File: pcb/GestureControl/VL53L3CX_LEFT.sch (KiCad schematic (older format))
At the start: 6 parts, among them U5 VL53L3CXV0DH_LEFT

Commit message: add
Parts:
- C12, C13: footprint Capacitor_SMD:C_0805_2012Metric_Pad1.18x1.45mm_HandSolder -> Capacitor_SMD:C_0603_1608Metric_Pad1.08x0.95mm_HandSolder
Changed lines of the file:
@@
 F 0 "C13" H 6915 3796 50  0000 L CNN
 F 1 "100n" H 6915 3705 50  0000 L CNN
-F 2 "Capacitor_SMD:C_0805_2012Metric_Pad1.18x1.45mm_HandSolder" H 6838 3600 50  0001 C CNN
+F 2 "Capacitor_SMD:C_0603_1608Metric_Pad1.08x0.95mm_HandSolder" H 6838 3600 50  0001 C CNN
 F 3 "~" H 6800 3750 50  0001 C CNN
 	1    6800 3750
@@
 F 0 "C12" H 3465 3796 50  0000 L CNN
 F 1 "100n" H 3465 3705 50  0000 L CNN
-F 2 "Capacitor_SMD:C_0805_2012Metric_Pad1.18x1.45mm_HandSolder" H 3388 3600 50  0001 C CNN
+F 2 "Capacitor_SMD:C_0603_1608Metric_Pad1.08x0.95mm_HandSolder" H 3388 3600 50  0001 C CNN
 F 3 "~" H 3350 3750 50  0001 C CNN
 	1    3350 3750

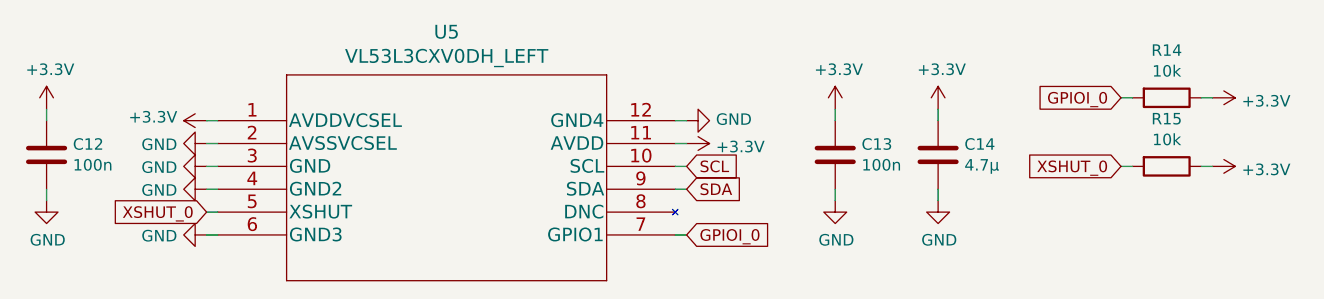
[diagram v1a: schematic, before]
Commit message: new PCB
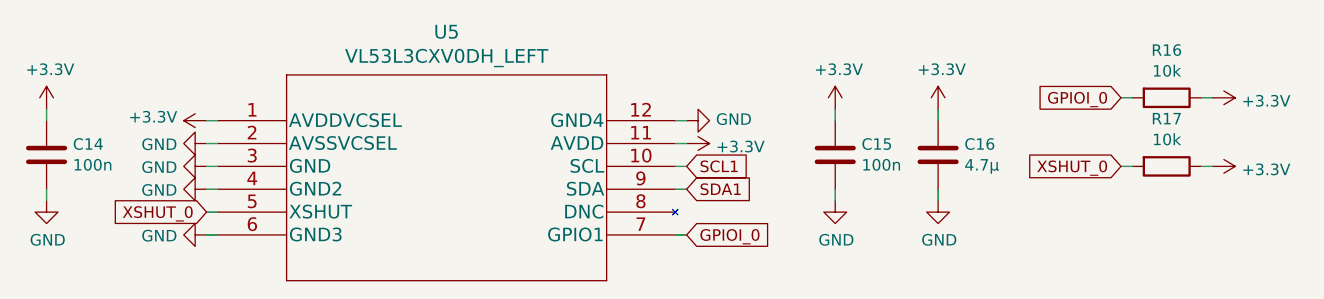
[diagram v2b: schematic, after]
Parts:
- U5: footprint VL53L3CX:VL53L3CXV0DH&slash_1 -> VL53L3C1:VL53L3CXV0DH&slash_1
- renumbered C12 to C14, C13 to C15, C14 to C16, R14 to R16, R15 to R17
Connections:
- net SCL renamed SCL1
- net SDA renamed SDA1
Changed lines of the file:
@@
 F 0 "U5" H 5100 3987 60  0000 C CNN
 F 1 "VL53L3CXV0DH_LEFT" H 5100 3881 60  0000 C CNN
-F 2 "VL53L3CX:VL53L3CXV0DH&slash_1" H 5100 3840 60  0001 C CNN
+F 2 "VL53L3C1:VL53L3CXV0DH&slash_1" H 5100 3840 60  0001 C CNN
 F 3 "" H 4100 3600 60  0000 C CNN
 	1    4100 3600
@@
 P 6150 3700
 AR Path="/62398514/623AF08A" Ref="#PWR?"  Part="1"
-AR Path="/623A3BAC/623AF08A" Ref="#PWR0147"  Part="1"
-F 0 "#PWR0147" H 6150 3550 50  0001 C CNN
+AR Path="/623A3BAC/623AF08A" Ref="#PWR059"  Part="1"
+F 0 "#PWR059" H 6150 3550 50  0001 C CNN
 F 1 "+3.3V" V 6165 3828 50  0000 L CNN
 F 2 "" H 6150 3700 50  0001 C CNN
@@
 P 6150 3600
 AR Path="/62398514/623AF090" Ref="#PWR?"  Part="1"
-AR Path="/623A3BAC/623AF090" Ref="#PWR0148"  Part="1"
-F 0 "#PWR0148" H 6150 3350 50  0001 C CNN
+AR Path="/623A3BAC/623AF090" Ref="#PWR058"  Part="1"
+F 0 "#PWR058" H 6150 3350 50  0001 C CNN
 F 1 "GND" V 6155 3472 50  0000 R CNN
 F 2 "" H 6150 3600 50  0001 C CNN
@@
 $EndComp
 Text GLabel 6150 3800 2    50   Input ~ 0
-SCL
+SCL1
 Text GLabel 6150 3900 2    50   Input ~ 0
-SDA
+SDA1
 $Comp
 L power:+3.3V #PWR?
@@
 P 4050 3600
 AR Path="/62398514/623AF098" Ref="#PWR?"  Part="1"
-AR Path="/623A3BAC/623AF098" Ref="#PWR0149"  Part="1"
-F 0 "#PWR0149" H 4050 3450 50  0001 C CNN
+AR Path="/623A3BAC/623AF098" Ref="#PWR053"  Part="1"
+F 0 "#PWR053" H 4050 3450 50  0001 C CNN
 F 1 "+3.3V" V 4065 3728 50  0000 L CNN
 F 2 "" H 4050 3600 50  0001 C CNN
@@
 P 4050 3800
 AR Path="/62398514/623AF09E" Ref="#PWR?"  Part="1"
-AR Path="/623A3BAC/623AF09E" Ref="#PWR0150"  Part="1"
-F 0 "#PWR0150" H 4050 3550 50  0001 C CNN
+AR Path="/623A3BAC/623AF09E" Ref="#PWR055"  Part="1"
+F 0 "#PWR055" H 4050 3550 50  0001 C CNN
 F 1 "GND" V 4055 3672 50  0000 R CNN
 F 2 "" H 4050 3800 50  0001 C CNN
@@
 P 4050 3900
 AR Path="/62398514/623AF0A4" Ref="#PWR?"  Part="1"
-AR Path="/623A3BAC/623AF0A4" Ref="#PWR0151"  Part="1"
-F 0 "#PWR0151" H 4050 3650 50  0001 C CNN
+AR Path="/623A3BAC/623AF0A4" Ref="#PWR056"  Part="1"
+F 0 "#PWR056" H 4050 3650 50  0001 C CNN
 F 1 "GND" V 4055 3772 50  0000 R CNN
 F 2 "" H 4050 3900 50  0001 C CNN
@@
 P 4050 4100
 AR Path="/62398514/623AF0AA" Ref="#PWR?"  Part="1"
-AR Path="/623A3BAC/623AF0AA" Ref="#PWR0152"  Part="1"
-F 0 "#PWR0152" H 4050 3850 50  0001 C CNN
+AR Path="/623A3BAC/623AF0AA" Ref="#PWR057"  Part="1"
+F 0 "#PWR057" H 4050 3850 50  0001 C CNN
 F 1 "GND" V 4055 3972 50  0000 R CNN
 F 2 "" H 4050 4100 50  0001 C CNN
@@
 P 4050 3700
 AR Path="/62398514/623AF0B1" Ref="#PWR?"  Part="1"
-AR Path="/623A3BAC/623AF0B1" Ref="#PWR0153"  Part="1"
-F 0 "#PWR0153" H 4050 3450 50  0001 C CNN
+AR Path="/623A3BAC/623AF0B1" Ref="#PWR054"  Part="1"
+F 0 "#PWR054" H 4050 3450 50  0001 C CNN
 F 1 "GND" V 4055 3572 50  0000 R CNN
 F 2 "" H 4050 3700 50  0001 C CNN
@@
 P 6800 3750
 AR Path="/62398514/623AF0C2" Ref="C?"  Part="1"
-AR Path="/623A3BAC/623AF0C2" Ref="C13"  Part="1"
-F 0 "C13" H 6915 3796 50  0000 L CNN
+AR Path="/623A3BAC/623AF0C2" Ref="C15"  Part="1"
+F 0 "C15" H 6915 3796 50  0000 L CNN
 F 1 "100n" H 6915 3705 50  0000 L CNN
 F 2 "Capacitor_SMD:C_0603_1608Metric_Pad1.08x0.95mm_HandSolder" H 6838 3600 50  0001 C CNN
@@
 P 7250 3750
 AR Path="/62398514/623AF0C8" Ref="C?"  Part="1"
-AR Path="/623A3BAC/623AF0C8" Ref="C14"  Part="1"
-F 0 "C14" H 7365 3796 50  0000 L CNN
+AR Path="/623A3BAC/623AF0C8" Ref="C16"  Part="1"
+F 0 "C16" H 7365 3796 50  0000 L CNN
 F 1 "4.7µ" H 7365 3705 50  0000 L CNN
 F 2 "Capacitor_SMD:C_0805_2012Metric_Pad1.18x1.45mm_HandSolder" H 7288 3600 50  0001 C CNN
@@
 P 6800 3550
 AR Path="/62398514/623AF0CE" Ref="#PWR?"  Part="1"
-AR Path="/623A3BAC/623AF0CE" Ref="#PWR0154"  Part="1"
-F 0 "#PWR0154" H 6800 3400 50  0001 C CNN
+AR Path="/623A3BAC/623AF0CE" Ref="#PWR060"  Part="1"
+F 0 "#PWR060" H 6800 3400 50  0001 C CNN
 F 1 "+3.3V" H 6815 3723 50  0000 C CNN
 F 2 "" H 6800 3550 50  0001 C CNN
@@
 P 7250 3550
 AR Path="/62398514/623AF0D4" Ref="#PWR?"  Part="1"
-AR Path="/623A3BAC/623AF0D4" Ref="#PWR0155"  Part="1"
-F 0 "#PWR0155" H 7250 3400 50  0001 C CNN
+AR Path="/623A3BAC/623AF0D4" Ref="#PWR062"  Part="1"
+F 0 "#PWR062" H 7250 3400 50  0001 C CNN
 F 1 "+3.3V" H 7265 3723 50  0000 C CNN
 F 2 "" H 7250 3550 50  0001 C CNN
@@
 P 6800 3950
 AR Path="/62398514/623AF0DA" Ref="#PWR?"  Part="1"
-AR Path="/623A3BAC/623AF0DA" Ref="#PWR0156"  Part="1"
-F 0 "#PWR0156" H 6800 3700 50  0001 C CNN
+AR Path="/623A3BAC/623AF0DA" Ref="#PWR061"  Part="1"
+F 0 "#PWR061" H 6800 3700 50  0001 C CNN
 F 1 "GND" H 6805 3777 50  0000 C CNN
 F 2 "" H 6800 3950 50  0001 C CNN
@@
 P 7250 3950
 AR Path="/62398514/623AF0E0" Ref="#PWR?"  Part="1"
-AR Path="/623A3BAC/623AF0E0" Ref="#PWR0157"  Part="1"
-F 0 "#PWR0157" H 7250 3700 50  0001 C CNN
+AR Path="/623A3BAC/623AF0E0" Ref="#PWR063"  Part="1"
+F 0 "#PWR063" H 7250 3700 50  0001 C CNN
 F 1 "GND" H 7255 3777 50  0000 C CNN
 F 2 "" H 7250 3950 50  0001 C CNN
@@
 P 8250 3800
 AR Path="/62398514/623AF0E6" Ref="R?"  Part="1"
-AR Path="/623A3BAC/623AF0E6" Ref="R15"  Part="1"
-F 0 "R15" V 8043 3800 50  0000 C CNN
+AR Path="/623A3BAC/623AF0E6" Ref="R17"  Part="1"
+F 0 "R17" V 8043 3800 50  0000 C CNN
 F 1 "10k" V 8134 3800 50  0000 C CNN
 F 2 "Resistor_SMD:R_0805_2012Metric_Pad1.20x1.40mm_HandSolder" V 8180 3800 50  0001 C CNN
@@
 P 8250 3500
 AR Path="/62398514/623AF0EC" Ref="R?"  Part="1"
-AR Path="/623A3BAC/623AF0EC" Ref="R14"  Part="1"
-F 0 "R14" V 8043 3500 50  0000 C CNN
+AR Path="/623A3BAC/623AF0EC" Ref="R16"  Part="1"
+F 0 "R16" V 8043 3500 50  0000 C CNN
 F 1 "10k" V 8134 3500 50  0000 C CNN
 F 2 "Resistor_SMD:R_0805_2012Metric_Pad1.20x1.40mm_HandSolder" V 8180 3500 50  0001 C CNN
@@
 P 8450 3500
 AR Path="/62398514/623AF0F4" Ref="#PWR?"  Part="1"
-AR Path="/623A3BAC/623AF0F4" Ref="#PWR0158"  Part="1"
-F 0 "#PWR0158" H 8450 3350 50  0001 C CNN
+AR Path="/623A3BAC/623AF0F4" Ref="#PWR064"  Part="1"
+F 0 "#PWR064" H 8450 3350 50  0001 C CNN
 F 1 "+3.3V" V 8465 3628 50  0000 L CNN
 F 2 "" H 8450 3500 50  0001 C CNN
@@
 P 8450 3800
 AR Path="/62398514/623AF0FA" Ref="#PWR?"  Part="1"
-AR Path="/623A3BAC/623AF0FA" Ref="#PWR0159"  Part="1"
-F 0 "#PWR0159" H 8450 3650 50  0001 C CNN
+AR Path="/623A3BAC/623AF0FA" Ref="#PWR065"  Part="1"
+F 0 "#PWR065" H 8450 3650 50  0001 C CNN
 F 1 "+3.3V" V 8465 3928 50  0000 L CNN
 F 2 "" H 8450 3800 50  0001 C CNN
@@
 P 3350 3750
 AR Path="/62398514/623AF108" Ref="C?"  Part="1"
-AR Path="/623A3BAC/623AF108" Ref="C12"  Part="1"
-F 0 "C12" H 3465 3796 50  0000 L CNN
+AR Path="/623A3BAC/623AF108" Ref="C14"  Part="1"
+F 0 "C14" H 3465 3796 50  0000 L CNN
 F 1 "100n" H 3465 3705 50  0000 L CNN
 F 2 "Capacitor_SMD:C_0603_1608Metric_Pad1.08x0.95mm_HandSolder" H 3388 3600 50  0001 C CNN
@@
 P 3350 3550
 AR Path="/62398514/623AF10E" Ref="#PWR?"  Part="1"
-AR Path="/623A3BAC/623AF10E" Ref="#PWR0160"  Part="1"
-F 0 "#PWR0160" H 3350 3400 50  0001 C CNN
+AR Path="/623A3BAC/623AF10E" Ref="#PWR051"  Part="1"
+F 0 "#PWR051" H 3350 3400 50  0001 C CNN
 F 1 "+3.3V" H 3365 3723 50  0000 C CNN
 F 2 "" H 3350 3550 50  0001 C CNN
@@
 P 3350 3950
 AR Path="/62398514/623AF114" Ref="#PWR?"  Part="1"
-AR Path="/623A3BAC/623AF114" Ref="#PWR0161"  Part="1"
-F 0 "#PWR0161" H 3350 3700 50  0001 C CNN
+AR Path="/623A3BAC/623AF114" Ref="#PWR052"  Part="1"
+F 0 "#PWR052" H 3350 3700 50  0001 C CNN
 F 1 "GND" H 3355 3777 50  0000 C CNN
 F 2 "" H 3350 3950 50  0001 C CNN

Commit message: add lib inside PCB
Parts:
- U5: footprint VL53L3C1:VL53L3CXV0DH&slash_1 -> VL53L3CX:VL53L3CXV0DH&slash_1
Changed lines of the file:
@@
 AR Path="/62398514/623AF083" Ref="U?"  Part="1"
 AR Path="/623A3BAC/623AF083" Ref="U5"  Part="1"
+AR Path="/623AF083" Ref="U5"  Part="1"
 F 0 "U5" H 5100 3987 60  0000 C CNN
 F 1 "VL53L3CXV0DH_LEFT" H 5100 3881 60  0000 C CNN
-F 2 "VL53L3C1:VL53L3CXV0DH&slash_1" H 5100 3840 60  0001 C CNN
+F 2 "VL53L3CX:VL53L3CXV0DH&slash_1" H 5100 3840 60  0001 C CNN
 F 3 "" H 4100 3600 60  0000 C CNN
 	1    4100 3600

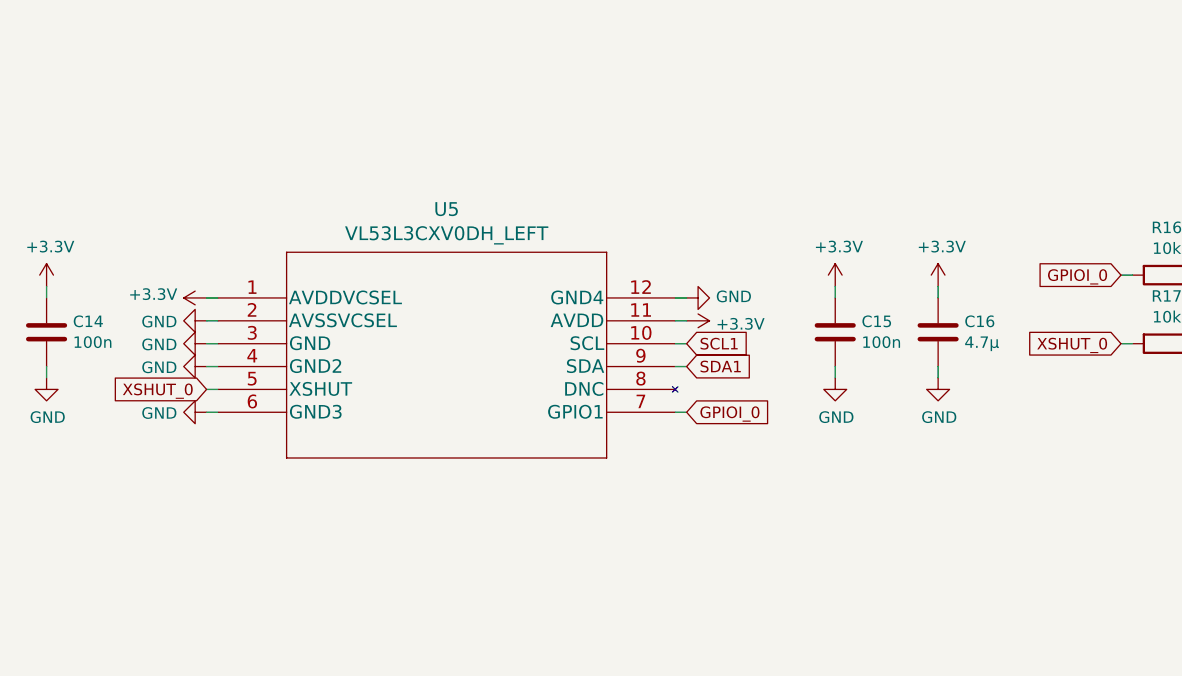
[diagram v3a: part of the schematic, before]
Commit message: add feedback Philip
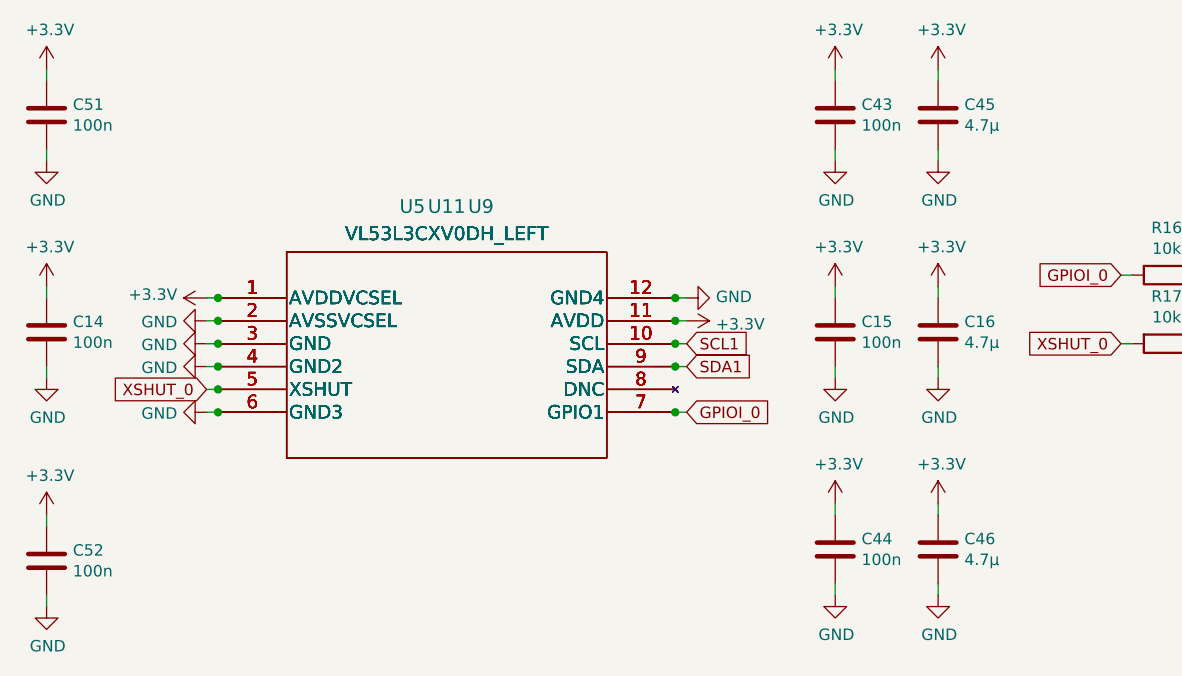
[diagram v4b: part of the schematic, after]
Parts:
- added C43, C44, C51, C52: 100n, Capacitor_SMD:C_0603_1608Metric_Pad1.08x0.95mm_HandSolder, symbol Device:C
- added C45, C46: 4.7µ, Capacitor_SMD:C_0805_2012Metric_Pad1.18x1.45mm_HandSolder, symbol Device:C
- added U11, U9: VL53L3CXV0DH_LEFT, VL53L3CX:VL53L3CXV0DH&slash_1, symbol VL53L3CX:VL53L3CXV0DH_1
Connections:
- net +3V3: now also C43.1, C44.1, C45.1, C46.1, C51.1, C52.1, U11.1 (AVDDVCSEL), U11.11 (AVDD), U9.1 (AVDDVCSEL), U9.11 (AVDD)
- net GND: now also C43.2, C44.2, C45.2, C46.2, C51.2, C52.2, U11.12 (GND4), U11.2 (AVSSVCSEL), U11.3 (GND), U11.4 (GND2), U11.6 (GND3), U9.12 (GND4), U9.2 (AVSSVCSEL), U9.3 (GND), U9.4 (GND2), U9.6 (GND3)
- net GPIOI_0: now also U11.7 (GPIO1), U9.7 (GPIO1)
- net SCL1: now also U11.10 (SCL), U9.10 (SCL)
- net SDA1: now also U11.9 (SDA), U9.9 (SDA)
- net XSHUT_0: now also U11.5 (XSHUT), U9.5 (XSHUT)
- net at U5.8 (DNC): now also U11.8 (DNC), U9.8 (DNC)

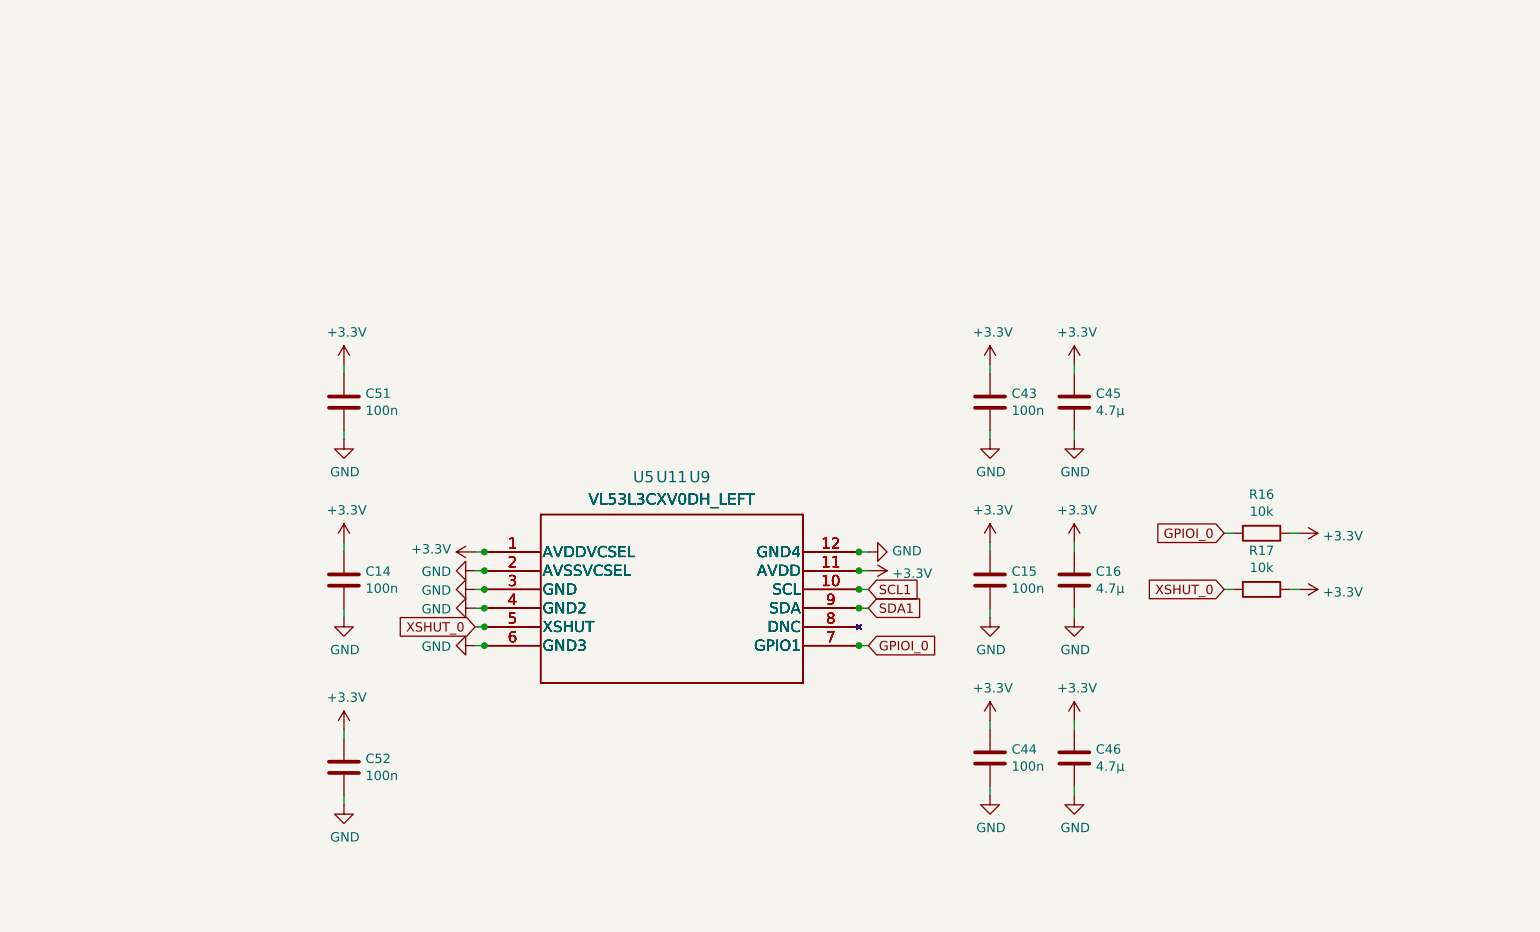
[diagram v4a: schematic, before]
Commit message: add PCBV0.11
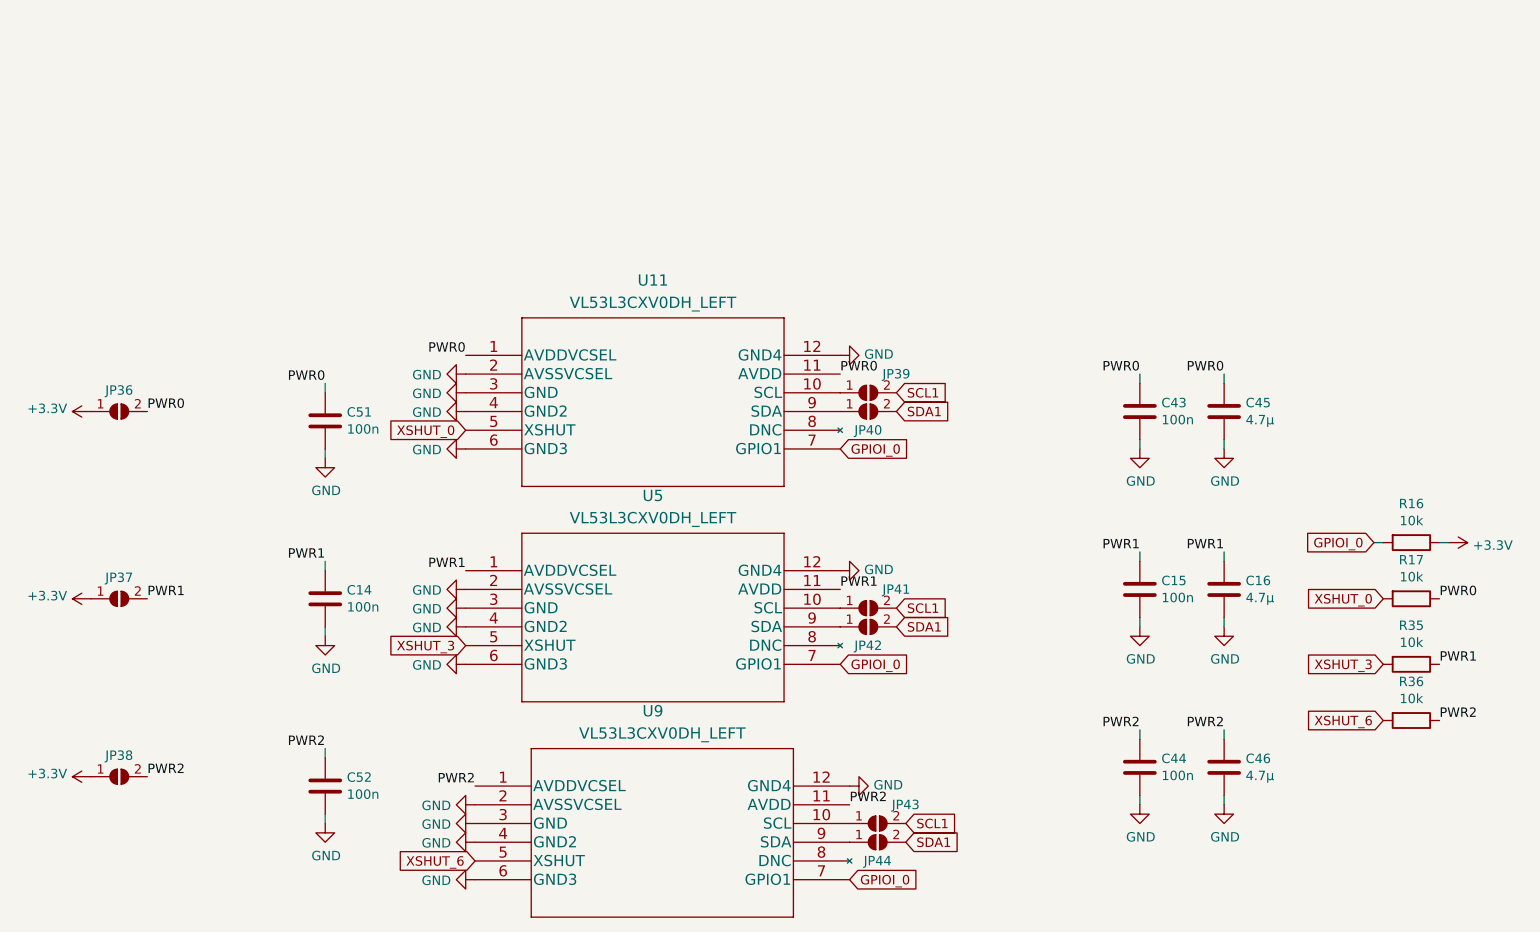
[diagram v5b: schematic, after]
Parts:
- added JP36, JP37, JP38, JP39, JP40, JP41, JP42, JP43, JP44: SolderJumper_2_Open, Jumper:SolderJumper-2_P1.3mm_Open_Pad1.0x1.5mm, symbol Jumper:SolderJumper_2_Open
- added R35, R36: 10k, Resistor_SMD:R_0805_2012Metric_Pad1.20x1.40mm_HandSolder, symbol Device:R
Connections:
- net +3V3: now also JP36.1 (A), JP37.1 (A), JP38.1 (A); no longer C14.1, C15.1, C16.1, C43.1, C44.1, C45.1, C46.1, C51.1, C52.1, R17.1, U11.1 (AVDDVCSEL), U11.11 (AVDD), U5.1 (AVDDVCSEL), U5.11 (AVDD), U9.1 (AVDDVCSEL), U9.11 (AVDD)
- net SCL1: now also JP39.2 (B), JP41.2 (B), JP43.2 (B); no longer U11.10 (SCL), U5.10 (SCL), U9.10 (SCL)
- net SDA1: now also JP40.2 (B), JP42.2 (B), JP44.2 (B); no longer U11.9 (SDA), U5.9 (SDA), U9.9 (SDA)
- net XSHUT_0: no longer U5.5 (XSHUT), U9.5 (XSHUT)
- new net: JP43.1 (A), U9.10 (SCL)
- new net: JP44.1 (A), U9.9 (SDA)
- new net: JP39.1 (A), U11.10 (SCL)
- new net: JP40.1 (A), U11.9 (SDA)
- new net: JP41.1 (A), U5.10 (SCL)
- new net: JP42.1 (A), U5.9 (SDA)
- new net PWR0: C43.1, C45.1, C51.1, JP36.2 (B), R17.1, U11.1 (AVDDVCSEL), U11.11 (AVDD)
- new net PWR1: C14.1, C15.1, C16.1, JP37.2 (B), R35.1, U5.1 (AVDDVCSEL), U5.11 (AVDD)
- new net PWR2: C44.1, C46.1, C52.1, JP38.2 (B), R36.1, U9.1 (AVDDVCSEL), U9.11 (AVDD)
- new net XSHUT_3: R35.2, U5.5 (XSHUT)
- new net XSHUT_6: R36.2, U9.5 (XSHUT)
- now unconnected: U11.8 (DNC), U5.8 (DNC), U9.8 (DNC)
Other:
- moved on the sheet: C14, C15, C16, C43, C44, C45, C46, C51, C52, R16, R17, U11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
